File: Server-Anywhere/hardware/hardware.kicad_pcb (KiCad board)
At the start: 2 copper layers, 57 x 63.7 mm, 9 parts, among them J1 power, J2 USB_C_Receptacle_USB2.0_16P

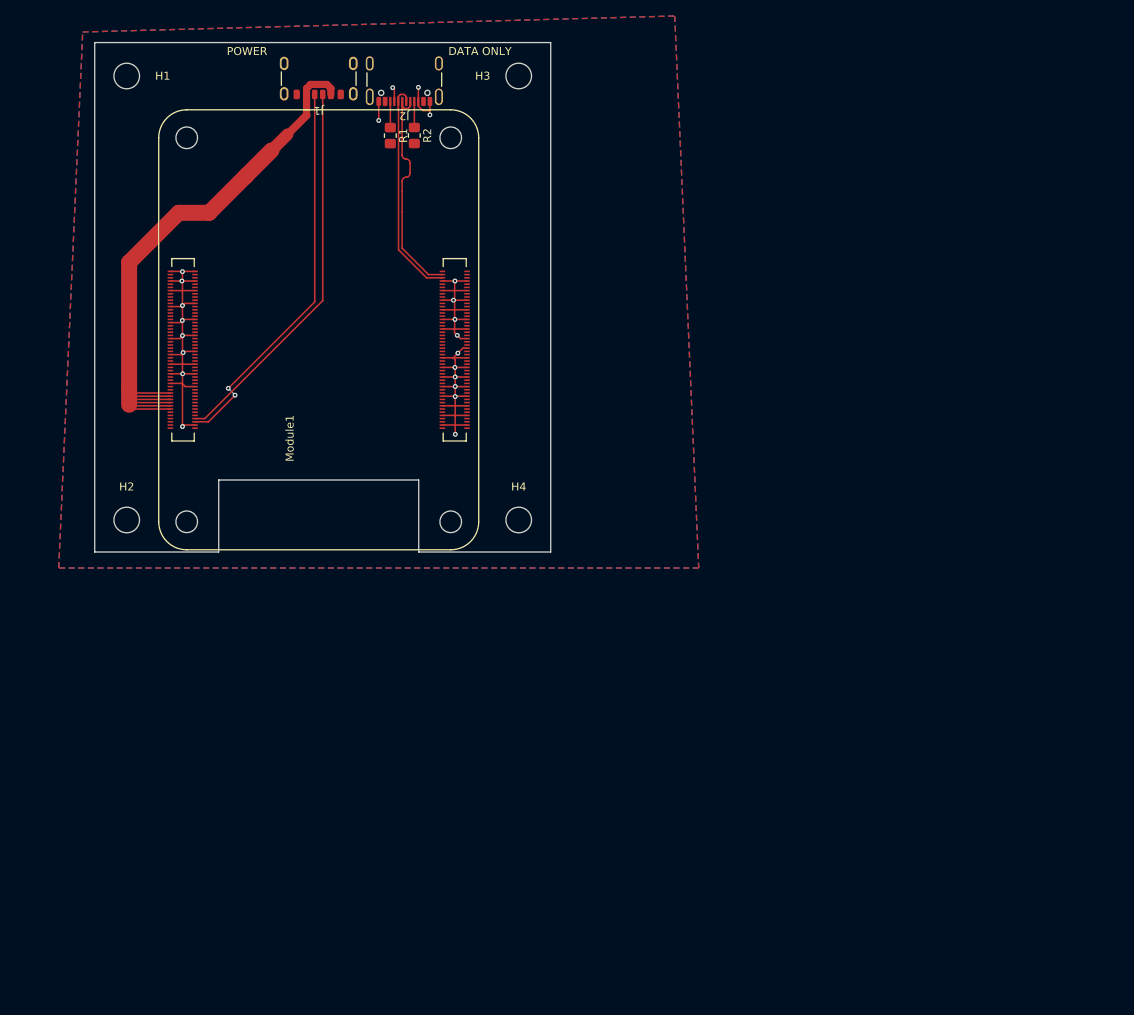
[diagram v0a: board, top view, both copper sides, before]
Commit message: yes
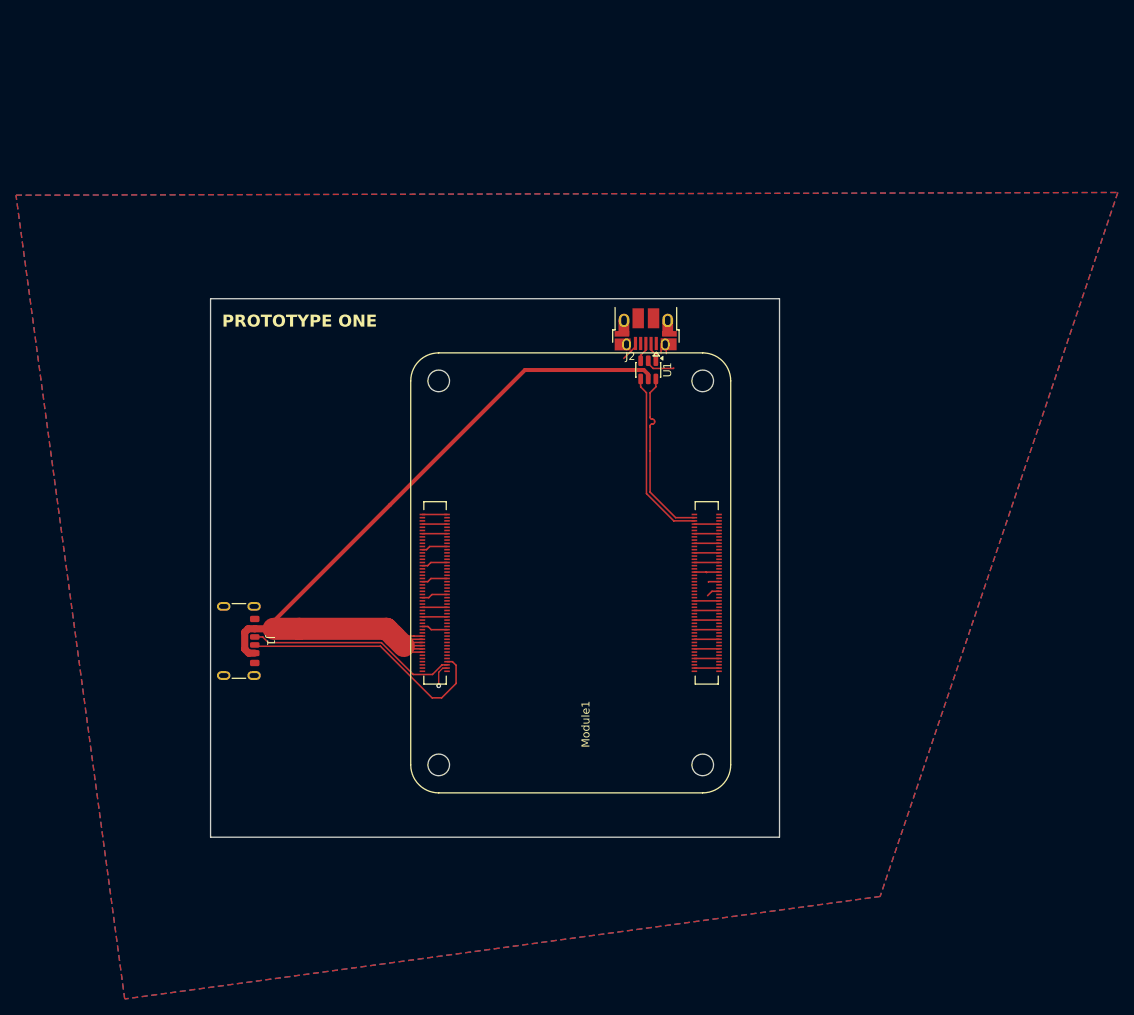
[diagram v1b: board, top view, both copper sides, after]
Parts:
- removed H1, H2, H3, H4: MountingHole, MountingHole:MountingHole_3.2mm_M3
- removed R1, R2: 5k1, Resistor_SMD:R_0805_2012Metric_Pad1.20x1.40mm_HandSolder
- added U1: USBLC6-4SC6, Package_TO_SOT_SMD:SOT-23-6, F.Cu at (148.7, 62.2)
- J1: value power -> USB_C_Receptacle_PowerOnly_6P
- J2: value USB_C_Receptacle_USB2.0_16P -> USB_OTG; footprint Connector_USB:USB_C_Receptacle_GCT_USB4105-xx-A_16P_TopMnt_Horizontal -> Connector_USB:USB_Micro-B_Amphenol_10103594-0001LF_Horizontal
- moved J1 72.2 mm to (96.4, 96.1), turned to -90 degrees
- moved J2 44.1 mm to (148.4, 57.2)
- moved Module1 43.8 mm to (122.5, 111.6)
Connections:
- net +5V renamed VBUS
- J1 pad A5: Net-(J1-CC1) -> /CC2
- J1 pad B5: Net-(J1-CC2) -> /CC1
- Module1 pad 103: USB_N -> /USB_N
- Module1 pad 105: USB_P -> /USB_P
- Module1 pad 94: Net-(J1-CC1) -> /CC1
- Module1 pad 96: Net-(J1-CC2) -> /CC2
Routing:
- net Net-(J1-CC2): track 48.8 -> 0.00 mm, vias 2 -> 0
- net Net-(J1-CC1): track 47.8 -> 0.00 mm
- net GND: track 125.9 -> 89.6 mm, vias 22 -> 1
- net /CC1: track 0.00 -> 32.2 mm
- net USB_N: track 28.3 -> 0.00 mm
- net USB_P: track 27.9 -> 0.00 mm
- net /CC2: track 0.00 -> 26.5 mm
- net /USB_P: track 0.00 -> 22.0 mm
- net /USB_N: track 0.00 -> 22.0 mm
- net VBUS: track 84.0 -> 99.5 mm
- net Net-(J2-CC2): track 3.27 -> 0.00 mm
- net Net-(J2-CC1): track 3.26 -> 0.00 mm
- net Net-(J2-D-): track 0.00 -> 2.40 mm
- net Net-(J2-D+): track 0.00 -> 2.40 mm
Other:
- board size 57 x 63.7 mm -> 71.1 x 67.3 mm
- board text added: "PROTOTYPE ONE"
- board text removed: "DATA ONLY"
- board text removed: "POWER"
- board text removed: "Server Anywhere v1"
